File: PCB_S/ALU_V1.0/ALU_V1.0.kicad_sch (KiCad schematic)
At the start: 532 parts, among them J1 Conn_01x08_Socket, J2 Conn_01x08_Socket, J3 Conn_01x08_Socket, J8 Conn_01x14_Pin, Q1 2N7002, Q10 2N7002, Q100 2N7002, Q101 2N7002, Q102 2N7002, Q103 2N7002, Q104 2N7002, Q105 2N7002, Q106 2N7002, Q107 2N7002, Q108 2N7002, Q109 2N7002, Q11 2N7002, Q110 2N7002, Q111 2N7002, Q112 2N7002, Q113 2N7002, Q114 2N7002, Q115 2N7002, Q116 2N7002, Q117 2N7002, Q118 2N7002, Q119 2N7002, Q12 2N7002, Q120 2N7002, Q121 2N7002, Q122 2N7002, Q123 2N7002, Q124 2N7002, Q125 2N7002, Q126 2N7002, Q127 2N7002, Q128 2N7002, Q129 2N7002, Q13 2N7002, Q130 2N7002, Q131 2N7002, Q132 2N7002, Q133 2N7002, Q134 2N7002, Q135 2N7002, Q136 2N7002, Q137 2N7002, Q138 2N7002, Q139 2N7002, Q14 2N7002, Q140 2N7002, Q141 2N7002, Q142 2N7002, Q143 2N7002, Q144 2N7002, Q145 2N7002, Q146 2N7002, Q147 2N7002, Q148 2N7002, Q149 2N7002, Q15 2N7002, Q150 2N7002, Q151 2N7002, Q152 2N7002, Q153 2N7002, Q154 2N7002, Q155 2N7002, Q156 2N7002, Q157 2N7002, Q158 2N7002, Q159 2N7002, Q16 2N7002, Q160 2N7002, Q161 2N7002, Q162 2N7002, Q163 2N7002, Q164 2N7002, Q165 2N7002, Q166 2N7002, Q167 2N7002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

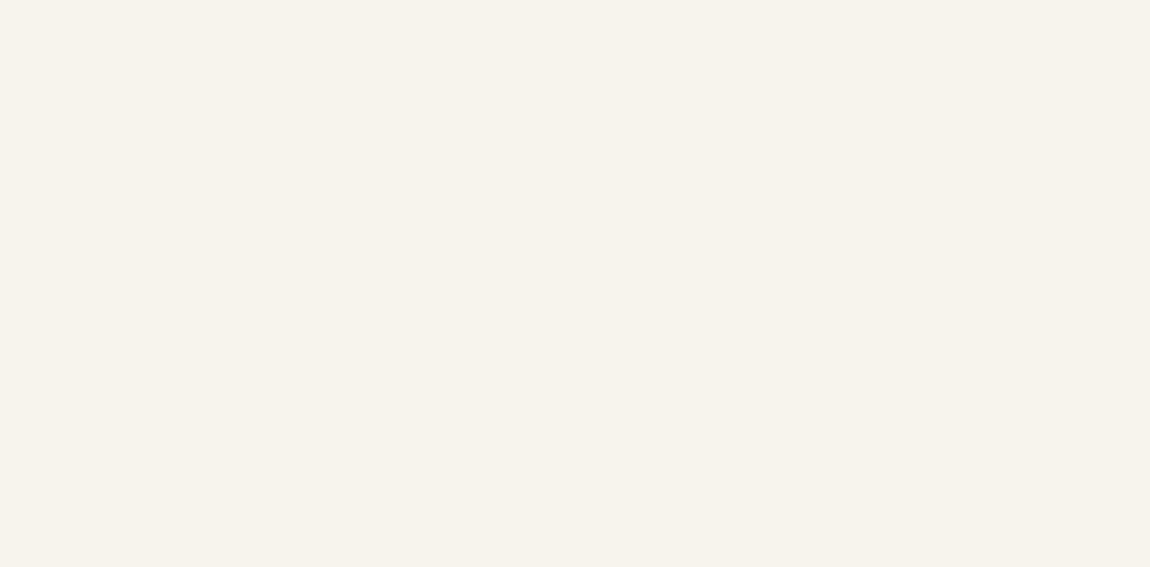
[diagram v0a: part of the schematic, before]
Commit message: ALU V1.0 more done
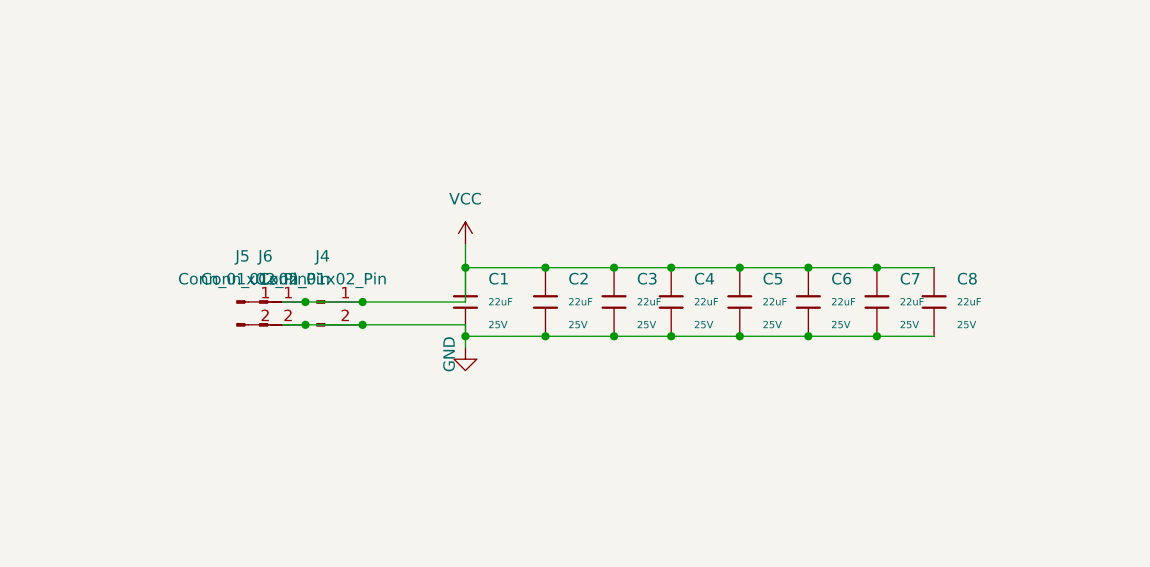
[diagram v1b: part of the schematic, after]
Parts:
- added C1, C2, C3, C4, C5, C6, C7, C8: 22uF, PCM_JLCPCB:C_0805, symbol PCM_JLCPCB-Capacitors:0805,22uF
- added J4, J5, J6: Conn_01x02_Pin, Connector_PinHeader_2.54mm:PinHeader_1x02_P2.54mm_Vertical, symbol Connector:Conn_01x02_Pin
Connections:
- net GND: now also C1.2, C2.2, C3.2, C4.2, C5.2, C6.2, C7.2, C8.2, J4.2 (Pin_2), J5.2 (Pin_2), J6.2 (Pin_2)
- net VCC: now also C1.1, C2.1, C3.1, C4.1, C5.1, C6.1, C7.1, C8.1, J4.1 (Pin_1), J5.1 (Pin_1), J6.1 (Pin_1)
